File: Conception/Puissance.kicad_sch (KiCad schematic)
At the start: 0 parts

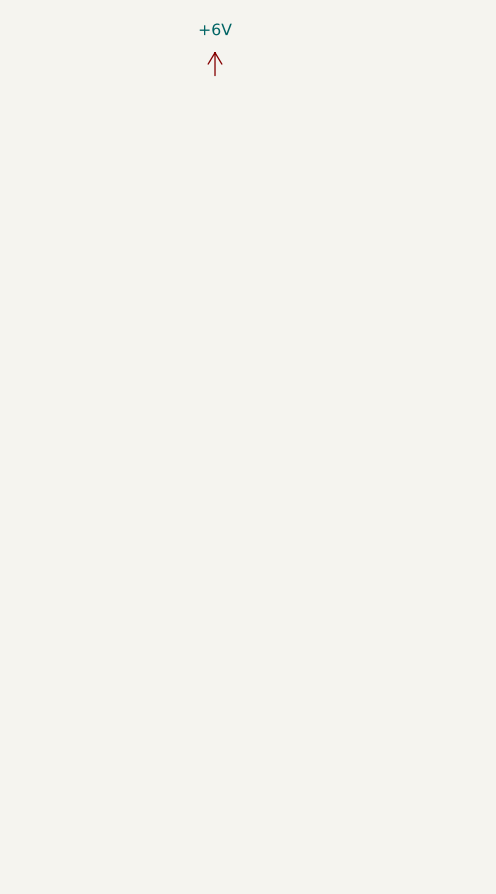
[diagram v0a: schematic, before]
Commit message: 1st drawing
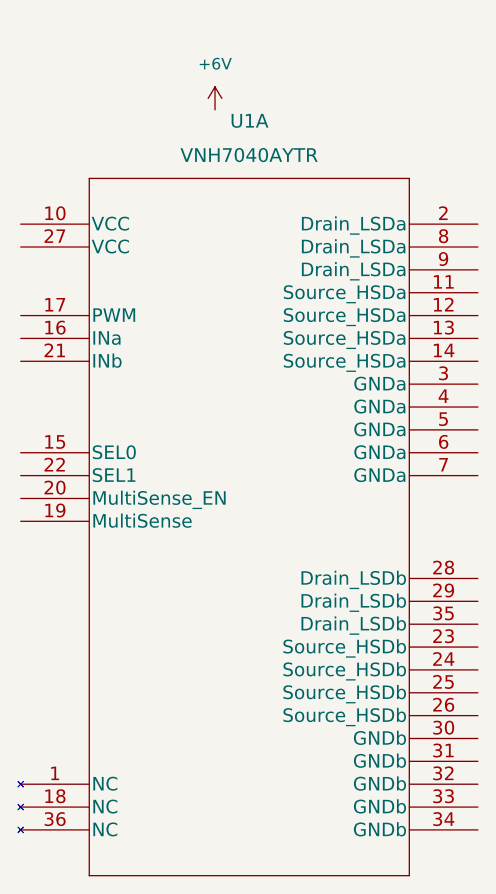
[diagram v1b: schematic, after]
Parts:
- added U1: VNH7040AYTR, Astromonkeys-footprints:VNH7040AYTR, symbol VNH7040AYTR:VNH7040AYTR
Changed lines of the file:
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@@
     (company "AstroMonkeys")
   )
-  (symbol (lib_id "power:+6V") (at 135.89 58.42 0) (unit 1)
+  (symbol (lib_id "power:+6V") (at 135.89 62.23 0) (unit 1)
     (in_bom yes) (on_board yes) (fields_autoplaced)
-    (property "Reference" "#PWR?" (id 0) (at 135.89 62.23 0)
+    (property "Reference" "#PWR02" (id 0) (at 135.89 66.04 0)
       (effects (font (size 1.27 1.27)) hide)
     )
-    (property "Value" "+6V" (id 1) (at 135.89 53.34 0))
-    (property "Footprint" "" (id 2) (at 135.89 58.42 0)
+    (property "Value" "+6V" (id 1) (at 135.89 57.15 0))
+    (property "Footprint" "" (id 2) (at 135.89 62.23 0)
       (effects (font (size 1.27 1.27)) hide)
     )
-    (property "Datasheet" "" (id 3) (at 135.89 58.42 0)
+    (property "Datasheet" "" (id 3) (at 135.89 62.23 0)
       (effects (font (size 1.27 1.27)) hide)
     )
     (pin "1")
   )
+  (symbol (lib_id "VNH7040AYTR:VNH7040AYTR") (at 114.3 77.47 0) (unit 1)
+    (in_bom yes) (on_board yes)
+    (property "Reference" "U1" (id 0) (at 139.7 63.5 0)
+      (effects (font (size 1.524 1.524)))
+    )
+    (property "Value" "VNH7040AYTR" (id 1) (at 139.7 67.31 0)
+      (effects (font (size 1.524 1.524)))
+    )
+    (property "Footprint" "Astromonkeys-footprints:VNH7040AYTR" (id 2) (at 139.7 67.31 0)
+      (effects (font (size 1.524 1.524)) hide)
+    )
+    (property "Datasheet" "" (id 3) (at 165.1 90.17 0)
+      (effects (font (size 1.524 1.524)))
+    )
+    (pin "1")
+    (pin "10")
+    (pin "11")
+    (pin "12")
+    (pin "13")
+    (pin "14")
+    (pin "15")
+    (pin "16")
+    (pin "17")
+    (pin "18")
+    (pin "19")
+    (pin "2")
+    (pin "20")
+    (pin "21")
+    (pin "22")
+    (pin "23")
+    (pin "24")
+    (pin "25")
+    (pin "26")
+    (pin "27")
+    (pin "28")
+    (pin "29")
+    (pin "3")
+    (pin "30")
+    (pin "31")
+    (pin "32")
+    (pin "33")
+    (pin "34")
+    (pin "35")
+    (pin "36")
+    (pin "4")
+    (pin "5")
+    (pin "6")
+    (pin "7")
+    (pin "8")
+    (pin "9")
+  )
 )
